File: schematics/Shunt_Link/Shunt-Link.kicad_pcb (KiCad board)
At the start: 2 copper layers, 17 parts, among them IC1 AD8221TRMZ-EP, IC2 AD8221TRMZ-EP, J1 PCIE-036-02-X-D-TH, J2 Conn_01x05_Socket

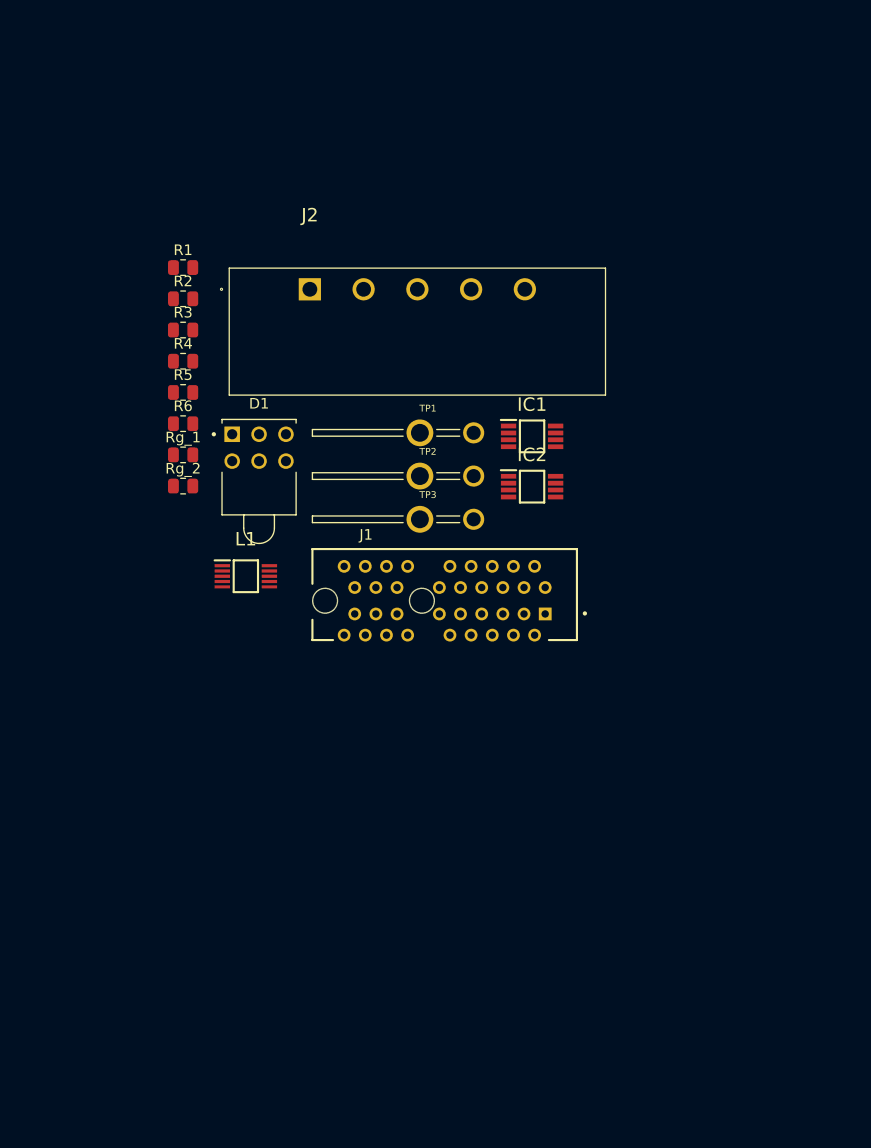
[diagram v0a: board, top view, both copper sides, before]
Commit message: Modifications to Shunt Link
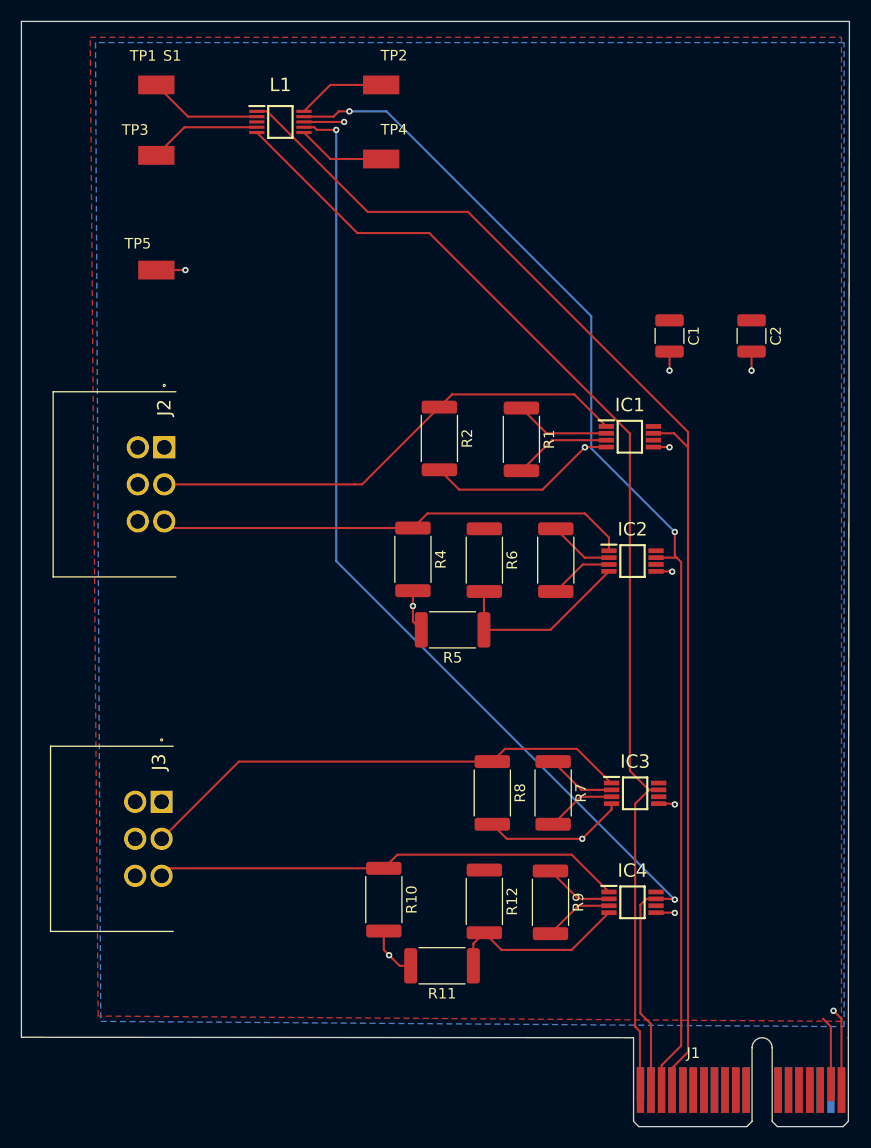
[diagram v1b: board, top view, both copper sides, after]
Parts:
- removed D1: WP130WCP_2EGW, Link_Footprints:LED_Lights
- removed Rg_1, Rg_2: 499, Resistor_SMD:R_0805_2012Metric
- added C1: 0.1 uF, Capacitor_SMD:C_1210_3225Metric, F.Cu at (138.8, 56.5)
- added C2: 10 uF, Capacitor_SMD:C_1210_3225Metric, F.Cu at (146.5, 56.5)
- added IC3: AD8221TRMZ-EP, Link_Footprints:AD8221TRMZ-EP, F.Cu at (135.5, 99.7)
- added IC4: AD8221TRMZ-EP, Link_Footprints:AD8221TRMZ-EP, F.Cu at (135.2, 110.0)
- added J3: Conn_02x03_Odd_Even, Link_Footprints:1818517, F.Cu at (90.8, 100.5)
- added R10: R, Resistor_SMD:R_2512_6332Metric, F.Cu at (111.8, 109.8)
- added R11: R, Resistor_SMD:R_2512_6332Metric, F.Cu at (117.2, 116.0)
- added R12: R, Resistor_SMD:R_2512_6332Metric, F.Cu at (121.2, 109.9)
- added R7: R_{g3}, Resistor_SMD:R_2512_6332Metric, F.Cu at (127.8, 99.7)
- added R8: R_{shunt}, Resistor_SMD:R_2512_6332Metric, F.Cu at (122.0, 99.7)
- added R9: R_{g4}, Resistor_SMD:R_2512_6332Metric, F.Cu at (127.5, 110.0)
- added TP4: T2, Link_Footprints:KEYSTONE_5017, F.Cu at (111.5, 39.8)
- added TP5: GND, Link_Footprints:KEYSTONE_5017, F.Cu at (90.2, 50.2)
- J1: footprint Link_Footprints:SAMTEC_PCIE_1x -> Connector_PCBEdge:BUS_PCIexpress_x1
- J2: value Conn_01x05_Socket -> Conn_02x03_Odd_Even; footprint Link_Footprints:Phoenix_Contact_MSTBA,5-LR -> Link_Footprints:1818517
- R1: value 6.25 -> R_{g1}; footprint Resistor_SMD:R_0805_2012Metric -> Resistor_SMD:R_2512_6332Metric
- R2: value 6.25 -> R_{shunt}; footprint Resistor_SMD:R_0805_2012Metric -> Resistor_SMD:R_2512_6332Metric
- R3: value 10.4 -> R_{g2}; footprint Resistor_SMD:R_0805_2012Metric -> Resistor_SMD:R_2512_6332Metric
- R4, R5: value 50 -> R; footprint Resistor_SMD:R_0805_2012Metric -> Resistor_SMD:R_2512_6332Metric
- R6: value 20.8 -> R; footprint Resistor_SMD:R_0805_2012Metric -> Resistor_SMD:R_2512_6332Metric
- TP1: value 1045 -> S1; footprint Link_Footprints:Keystone_1045 -> Link_Footprints:KEYSTONE_5017
- TP2: value 1045 -> T1; footprint Link_Footprints:Keystone_1045 -> Link_Footprints:KEYSTONE_5017
- TP3: value 1045 -> S2; footprint Link_Footprints:Keystone_1045 -> Link_Footprints:KEYSTONE_5017
- moved J1 50.4 mm to (136.0, 127.8)
- moved L1 43.1 mm to (102.0, 36.2)
- moved TP3 42.5 mm to (90.2, 39.4)
- moved R3 41.4 mm to (128.0, 77.7), turned to -90 degrees
- moved TP1 41.3 mm to (90.2, 32.8)
- moved TP2 37.1 mm to (111.5, 32.8)
- moved R1 35.9 mm to (124.8, 66.2), turned to -90 degrees
- moved R5 33.9 mm to (118.2, 84.2), turned to 180 degrees
- moved R6 31.3 mm to (121.2, 77.7), turned to -90 degrees
- moved R4 28.7 mm to (114.5, 77.6), turned to -90 degrees
- moved R2 27.6 mm to (117.0, 66.2), turned to -90 degrees
- moved J2 20.3 mm to (91.0, 67.0), turned to -90 degrees
- moved IC2 11.8 mm to (135.2, 77.8)
- moved IC1 9.24 mm to (135.0, 66.0)
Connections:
- IC1 pad 1: /S_{+} -> /S_{1+}
- IC1 pad 4: /GND -> GND
- IC1 pad 5: /GND -> GND
- IC1 pad 6: /V_{ref} -> /+2V5
- IC1 pad 7: /S_{o} -> /S_{1out}
- IC1 pad 8: /V_{s} -> +12V
- IC2 pad 1: /T_{+} -> /T_{1-}
- IC2 pad 4: /GND -> Net-(IC2-+IN)
- IC2 pad 5: /GND -> GND
- IC2 pad 7: /T_{o} -> /T_{1out}
- IC2 pad 8: /V_{s} -> unconnected-(IC2-+VS-Pad8)
- J1 pad A1: /NC -> unconnected-(J1-PadA1)
- J1 pad A10: /NC -> unconnected-(J1-PadA10)
- J1 pad A11: /NC -> unconnected-(J1-PadA11)
- J1 pad A12: /NC -> unconnected-(J1-PadA12)
- J1 pad A13: /NC -> unconnected-(J1-PadA13)
- J1 pad A14: /NC -> unconnected-(J1-PadA14)
- J1 pad A15: /NC -> unconnected-(J1-PadA15)
- J1 pad A16: /NC -> unconnected-(J1-PadA16)
- J1 pad A17: /NC -> unconnected-(J1-PadA17)
- J1 pad A18: /NC -> unconnected-(J1-PadA18)
- J1 pad A2: /NC -> unconnected-(J1-PadA2)
- J1 pad A3: /NC -> unconnected-(J1-PadA3)
- J1 pad A4: /NC -> unconnected-(J1-PadA4)
- J1 pad A5: /NC -> unconnected-(J1-PadA5)
- J1 pad A6: /NC -> unconnected-(J1-PadA6)
- J1 pad A7: /NC -> unconnected-(J1-PadA7)
- J1 pad A8: /NC -> unconnected-(J1-PadA8)
- J1 pad A9: /NC -> unconnected-(J1-PadA9)
- J1 pad B1: /S_{o} -> /S_{2out}
- J1 pad B10: /Green_{1} -> unconnected-(J1-PadB10)
- J1 pad B11: /Red_{1} -> unconnected-(J1-PadB11)
- J1 pad B12: /Green_{2} -> unconnected-(J1-PadB12)
- J1 pad B13: /Red_{2} -> unconnected-(J1-PadB13)
- J1 pad B14: /NC -> unconnected-(J1-PadB14)
- J1 pad B15: /NC -> unconnected-(J1-PadB15)
- J1 pad B16: /NC -> unconnected-(J1-PadB16)
- J1 pad B17: /V_{s} -> +12V
- J1 pad B18: /GND -> GND
- J1 pad B2: /T_{o} -> /T_{2out}
- J1 pad B3: /NC -> /T_{1out}
- J1 pad B4: /NC -> /S_{1out}
- J1 pad B5: /NC -> unconnected-(J1-PadB5)
- J1 pad B6: /NC -> unconnected-(J1-PadB6)
- J1 pad B7: /NC -> unconnected-(J1-PadB7)
- J1 pad B8: /NC -> unconnected-(J1-PadB8)
- J1 pad B9: /NC -> unconnected-(J1-PadB9)
- J2 pad 1: /GND -> +12V
- J2 pad 2: /V_{+} -> /S_{1+}
- J2 pad 3: /T_{+} -> /T_{1-}
- J2 pad 4: /V_{+} -> +12V
- J2 pad 5: /S_{+} -> unconnected-(J2-Pin_5-Pad5)
- L1 pad 1: /V_{2.5} -> /S_{1out}
- L1 pad 10: /T_{o} -> /T_{1test}
- L1 pad 2: /V_{ref} -> /S_{1test}
- L1 pad 3: /V_{s} -> +12V
- L1 pad 4: /V_{+} -> /S_{2test}
- L1 pad 5: /V_{5} -> /S_{2out}
- L1 pad 6: /S_{o} -> /T_{2test}
- L1 pad 7: /S_{test} -> /T_{2out}
- L1 pad 8: /GND -> GND
- L1 pad 9: /T_{test} -> /T_{1out}
- R1 pad 1: /S_{+} -> Net-(IC1-RG_1)
- R1 pad 2: /GND -> Net-(IC1-RG_2)
- R2 pad 1: /T_{+} -> /S_{1+}
- R2 pad 2: /GND -> GND
- R3 pad 1: /V_{2.5} -> Net-(IC2-RG_1)
- R3 pad 2: /GND -> Net-(IC2-RG_2)
- R4 pad 1: /V_{s} -> /T_{1-}
- R4 pad 2: /V_{2.5} -> GND
- R5 pad 1: /V_{s} -> Net-(IC2-+IN)
- R5 pad 2: /V_{5} -> GND
- R6 pad 1: /V_{5} -> +12V
- R6 pad 2: /GND -> Net-(IC2-+IN)
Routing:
- net /S_{1out}: track 0.00 -> 119.9 mm
- net /T_{1out}: track 0.00 -> 114.8 mm, vias 0 -> 2
- net /S_{2out}: track 0.00 -> 112.4 mm
- net /T_{2out}: track 0.00 -> 110.6 mm, vias 0 -> 2
- net GND: track 0.00 -> 65.4 mm, vias 0 -> 13
- net /S_{2+}: track 0.00 -> 47.4 mm
- net /S_{1+}: track 0.00 -> 46.5 mm
- net /T_{1-}: track 0.00 -> 45.0 mm
- net /T_{2-}: track 0.00 -> 44.6 mm
- net Net-(IC2-+IN): track 0.00 -> 17.7 mm
- net Net-(IC4-+IN): track 0.00 -> 17.5 mm
- net /S_{1test}: track 0.00 -> 10.7 mm
- net /S_{2test}: track 0.00 -> 10.6 mm
- net Net-(IC1-RG_2): track 0.00 -> 9.22 mm
- net Net-(IC1-RG_1): track 0.00 -> 9.14 mm
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- added copper zone on F.Cu, net +12V
- added copper zone on B.Cu, net GND
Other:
- board outline added: 78.2 x 96 mm
- board text added: "OATS Center Shunt-Link v1 (10/13/2025) abalmos@purdue.edu"
